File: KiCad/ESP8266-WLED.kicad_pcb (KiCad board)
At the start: 2 copper layers, 25.4 x 40.7 mm, 33 parts, among them J1 USB_C_Receptacle_USB2.0_14P, J2 Conn_01x01_Socket, J3 Conn_01x01_Socket, J4 Conn_01x01_Socket, J5 Conn_01x01_Socket, SW1 SW_Push, SW2 SW_Push, U1 ESP-12F, U2 MIC5219-3.3YM5

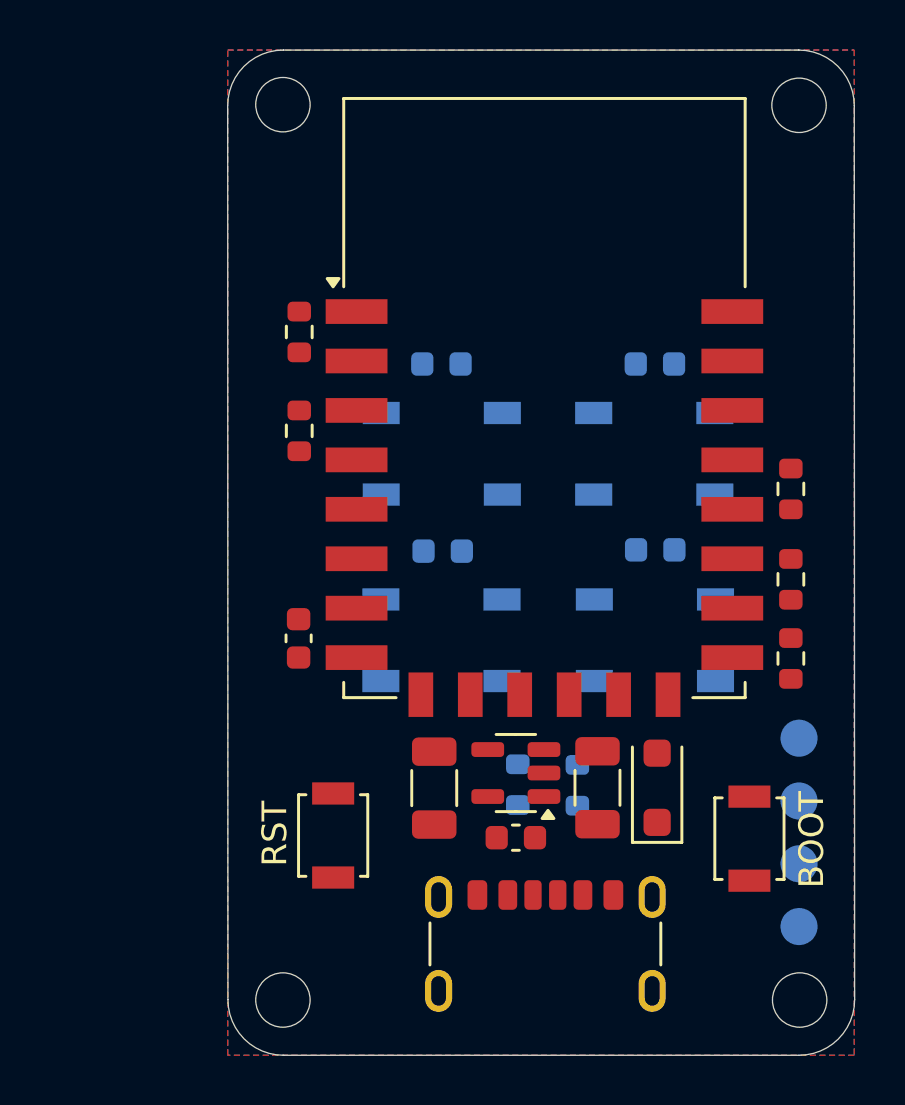
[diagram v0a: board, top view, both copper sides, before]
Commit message: first placement
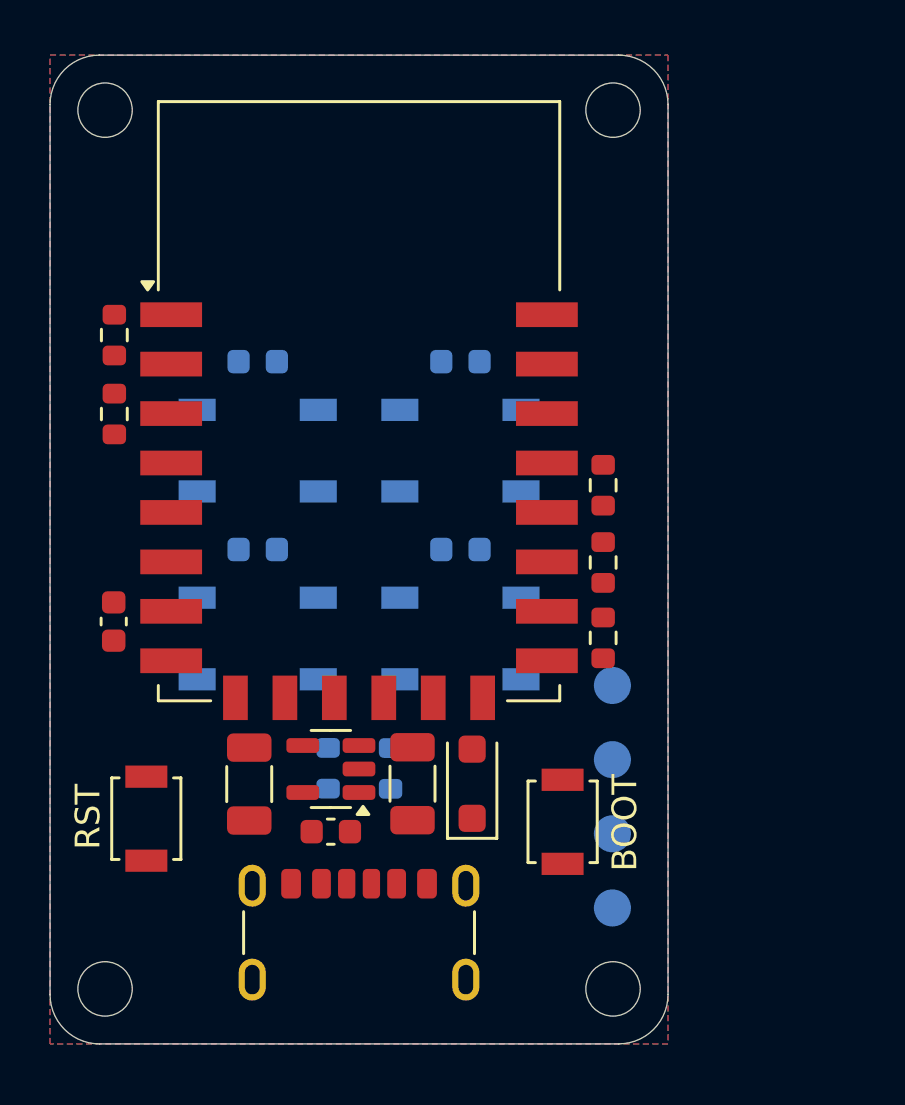
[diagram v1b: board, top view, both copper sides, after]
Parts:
- moved C3 7.88 mm to (146.6, 104.0)
- moved C2 7.87 mm to (146.6, 96.4)
- moved D3 7.87 mm to (146.6, 107.6)
- moved J2 7.84 mm to (152.8, 109.5)
- moved D1 7.84 mm to (146.6, 100.0)
- moved J3 7.73 mm to (152.8, 112.5)
- moved R6 7.70 mm to (141.2, 112.8)
- moved J4 7.65 mm to (152.8, 115.5)
- moved R5 7.64 mm to (152.4, 107.6)
- moved R4 7.62 mm to (152.4, 104.5)
- moved R3 7.60 mm to (152.4, 101.4)
- moved R7 7.59 mm to (143.8, 112.9)
- moved SW1 7.59 mm to (150.7, 115.0)
- moved SW2 7.59 mm to (133.9, 114.9)
- moved J5 7.59 mm to (152.8, 118.5)
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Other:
- board size 25.4 x 40.7 mm -> 25 x 40 mm
- board text added: "https://github.com/dokuhn/ESP8266-WLED"
